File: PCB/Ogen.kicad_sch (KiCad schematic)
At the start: 17 parts, among them J1 Input, U1 PMW3360DM-T2QU, U2 TLV70019, U3 TXS0102DCU, U4 TXS0102DCU, U5 TXS0102DCU

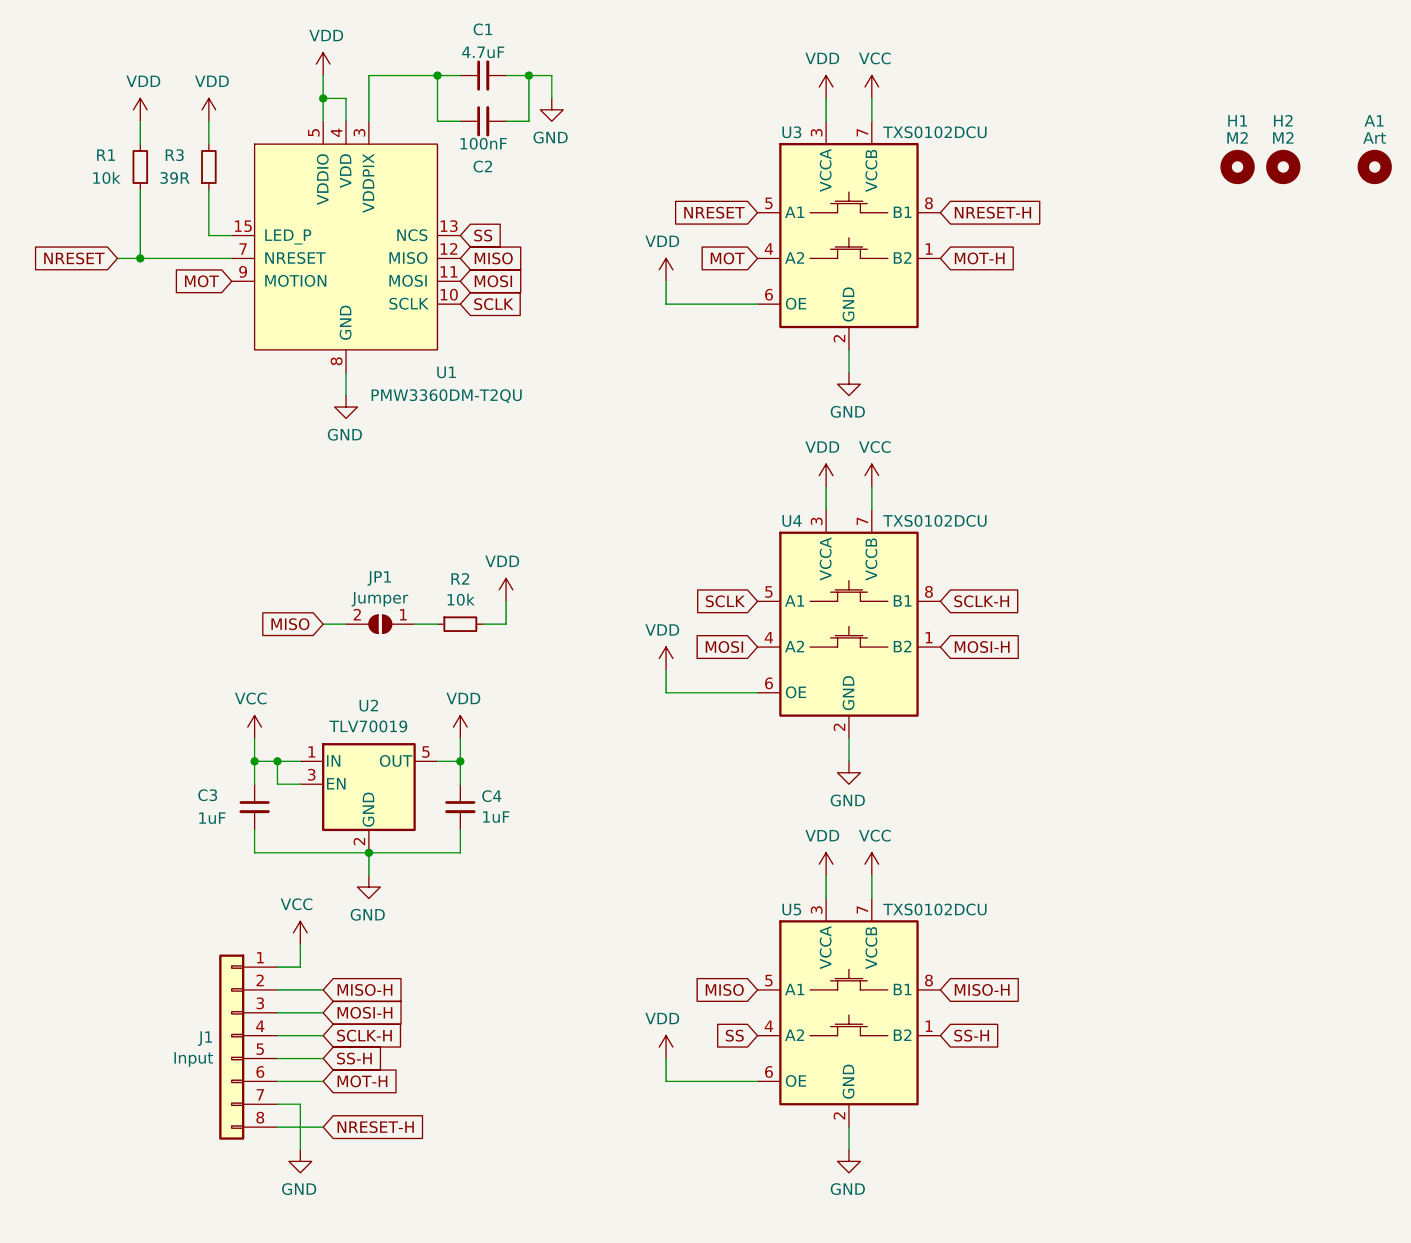
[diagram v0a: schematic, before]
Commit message: V1.2 update.
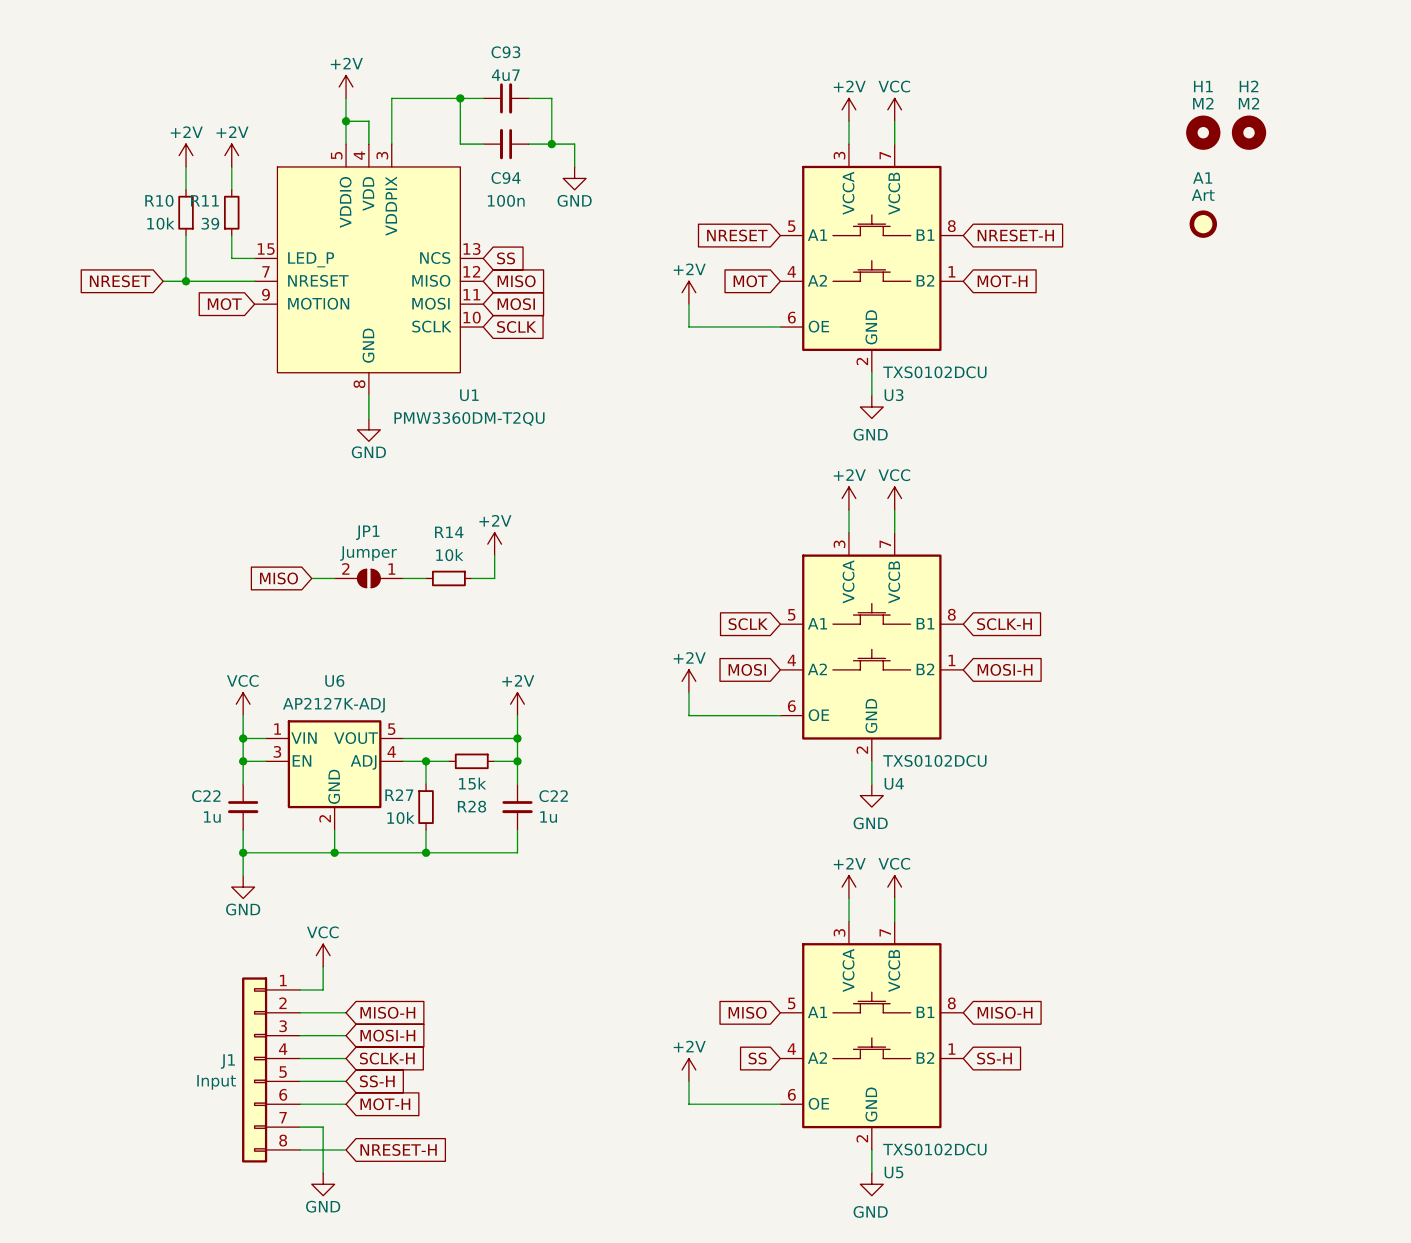
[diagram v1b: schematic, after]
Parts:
- removed C1: 4.7uF, Capacitor_SMD:C_0603_1608Metric, symbol Device:C_Small
- removed C2: 100nF, Capacitor_SMD:C_0603_1608Metric, symbol Device:C_Small
- removed C3, C4: 1uF, Capacitor_SMD:C_0603_1608Metric, symbol Device:C_Small
- removed R1, R2: 10k, Resistor_SMD:R_0603_1608Metric, symbol Device:R_Small
- removed R3: 39R, Resistor_SMD:R_0603_1608Metric, symbol Device:R_Small
- removed U2: TLV70019, Package_TO_SOT_SMD:SOT-23-5, symbol Regulator_Linear:TLV70019_SOT23-5
- added C22 (x2): 1u, Capacitor_SMD:C_0402_1005Metric, symbol Device:C_Small
- added C93: 4u7, Capacitor_SMD:C_0603_1608Metric, symbol Device:C_Small
- added C94: 100n, Capacitor_SMD:C_0402_1005Metric, symbol Device:C_Small
- added R10, R14, R27: 10k, Resistor_SMD:R_0402_1005Metric, symbol Device:R_Small
- added R11: 39, Resistor_SMD:R_0402_1005Metric, symbol Device:R_Small
- added R28: 15k, Resistor_SMD:R_0402_1005Metric, symbol Device:R_Small
- added U6: AP2127K-ADJ, Package_TO_SOT_SMD:SOT-23-5, symbol Regulator_Linear:AP2127K-ADJ
- A1: footprint Ogen:Ariamelon_Logo -> Ogen:Ariamelon_Logo-CU; symbol Mechanical:MountingHole -> Mechanical:Fiducial
- U3, U4, U5: LCSC (none) -> C53434
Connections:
- net GND: now also C22.2, C22.2, C93.2, C94.1, R27.2, U6.2 (GND)
- net NRESET: now also R10.1
- net VCC: now also C22.1, U6.1 (VIN), U6.3 (EN)
- net at U1.3 (VDDPIX): now also C93.1, C94.2
- net at U1.15 (LED_P): now also R11.1
- net at JP1.1 (A): now also R14.2
- net VDD renamed +2V
- net +2V: now also C22.1, R10.2, R11.2, R14.1, R28.1, U6.5 (VOUT)
- new net: R27.1, R28.2, U6.4 (ADJ)
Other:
- moved on the sheet: H1, H2, J1, JP1, U1, U3, U4, U5
